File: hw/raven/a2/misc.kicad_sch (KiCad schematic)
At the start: 71 parts, among them J601 TRSx2, J602 PinHdr_01x04, J603 PinHdr_01x04, J604 PinHdr_01x04, J605 Pinhdr_01x02, J606 DB25/9/9, J607 PinHdr_01x04, J608 DB9M/9M, J609 USB+Ethernet, U601 MCP4251, U602 PAM8302AAD, U603 CNY17F-3, U604 74LS07

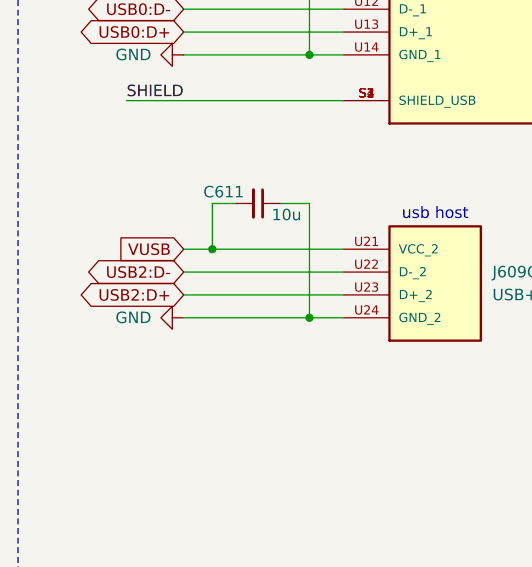
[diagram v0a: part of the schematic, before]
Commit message: more a2 wip
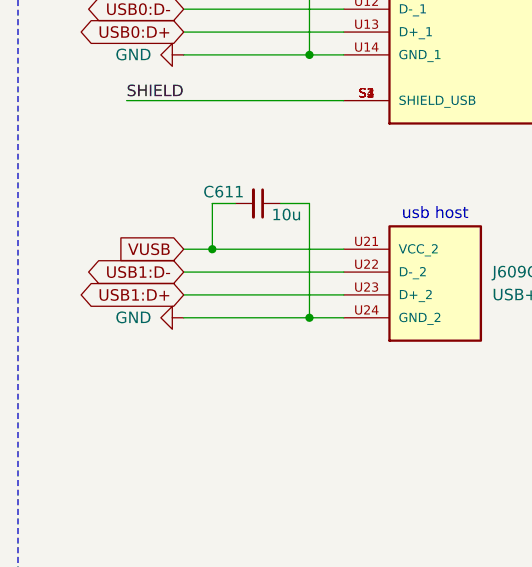
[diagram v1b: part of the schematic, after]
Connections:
- net USB2:D+ renamed USB1:D+
- net USB2:D- renamed USB1:D-
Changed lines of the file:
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@@
 		)
 	)
-	(global_label "USB2:D-"
+	(global_label "USB1:D-"
 		(shape bidirectional)
 		(at 34.29 205.74 180)
@@
 		)
 	)
-	(global_label "USB2:D+"
+	(global_label "USB1:D+"
 		(shape bidirectional)
 		(at 34.29 208.28 180)
